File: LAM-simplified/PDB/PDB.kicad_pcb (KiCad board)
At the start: 2 copper layers, 115 x 115 mm, 22 parts, among them J1 Conn_02x03_Counter_Clockwise, J10 Conn_01x02, J11 Conn_01x02, J12 Conn_01x02, J13 Conn_01x02, J14 Conn_01x02, J15 Conn_01x02, J16 Conn_01x02, J2 Conn_02x03_Counter_Clockwise, J3 Conn_02x03_Counter_Clockwise, J4 Conn_02x03_Counter_Clockwise, J5 Conn_01x02, J6 Conn_01x02, J7 Conn_01x02, J8 Conn_01x02, J9 Conn_01x02

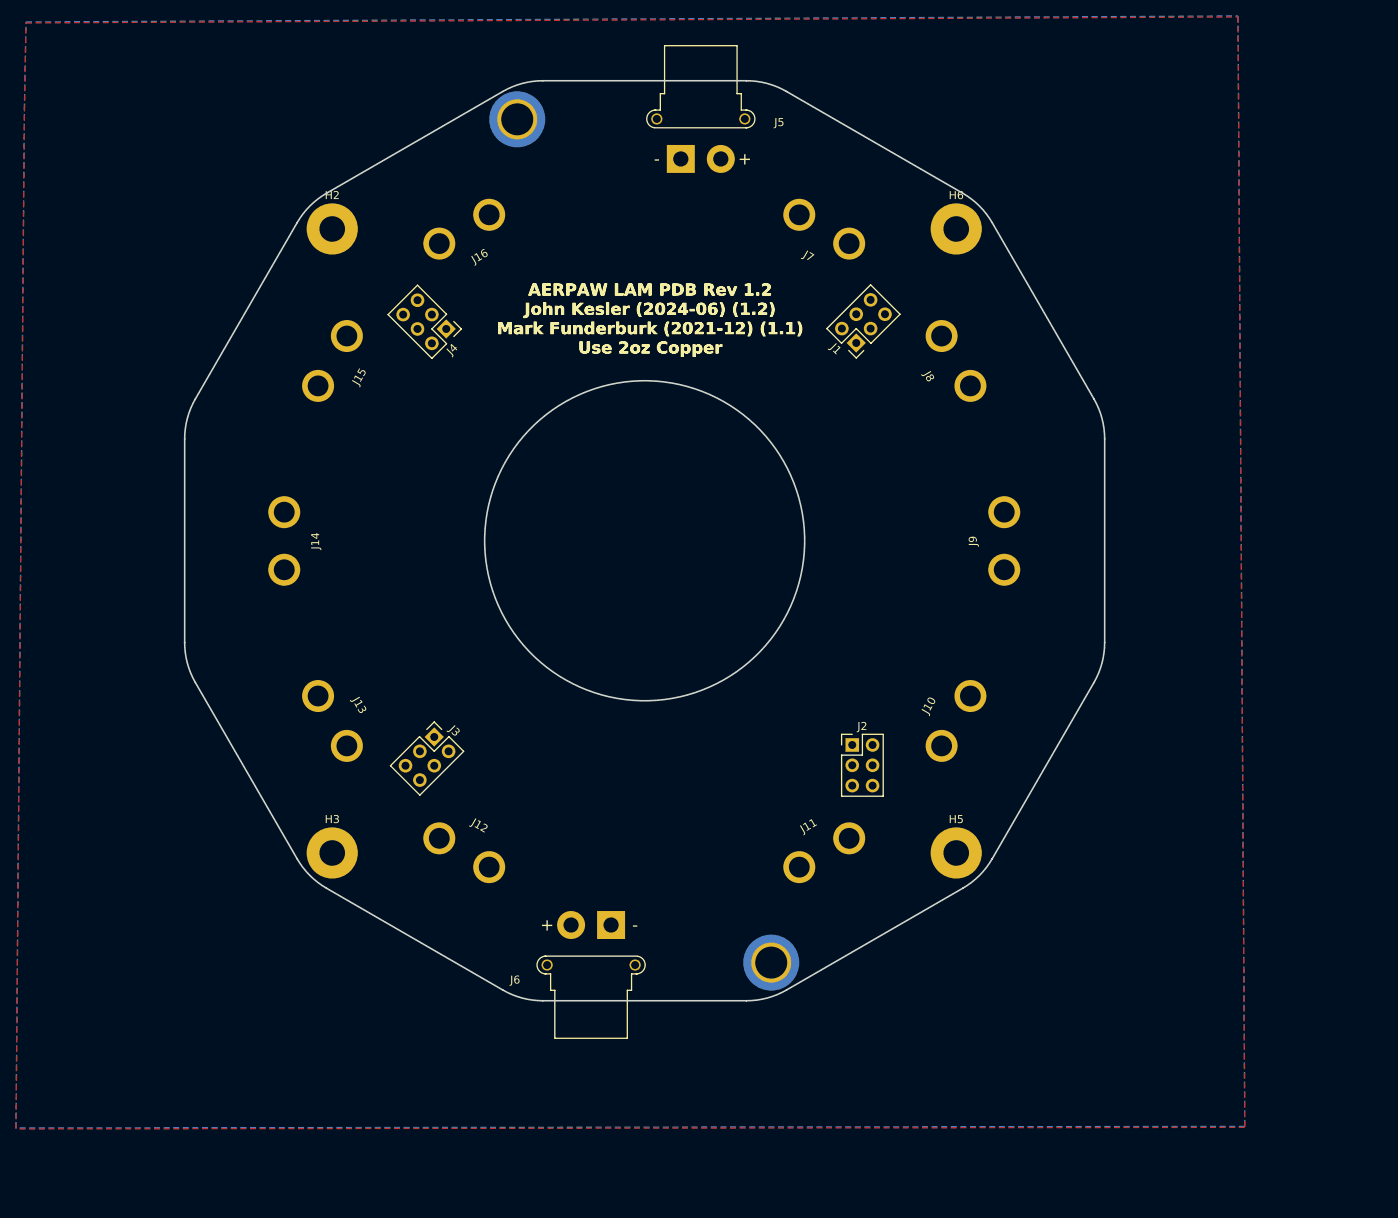
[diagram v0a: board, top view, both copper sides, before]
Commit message: update LAM PDB PCB r1.3
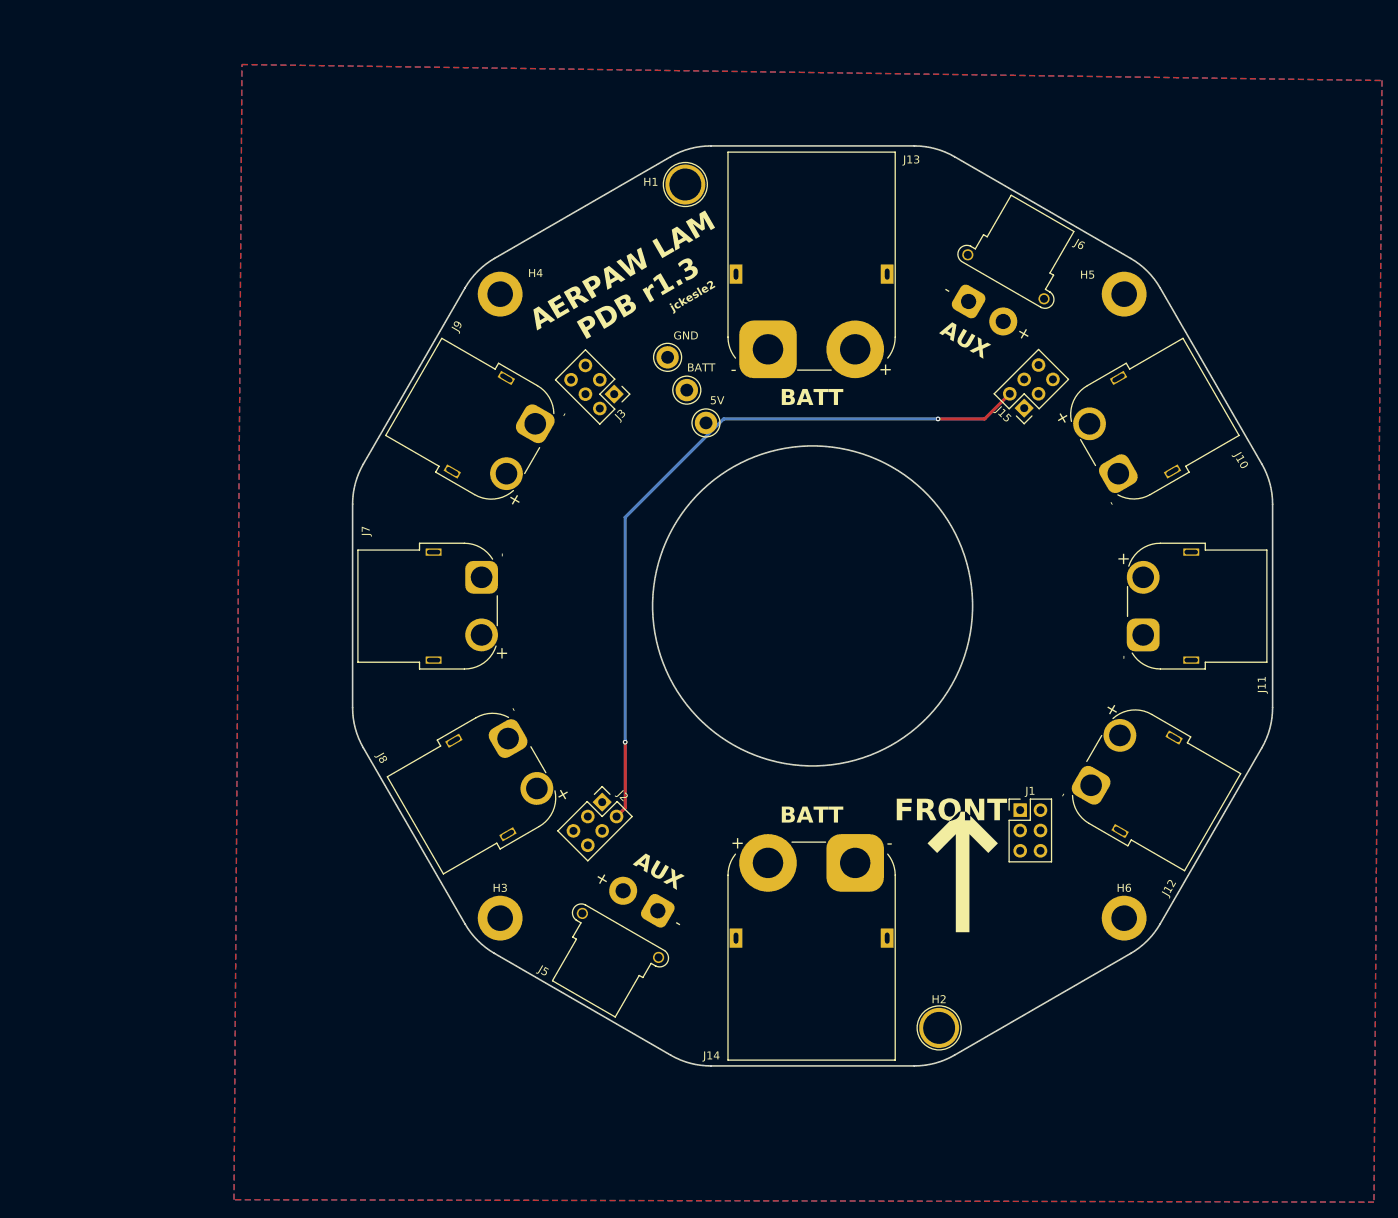
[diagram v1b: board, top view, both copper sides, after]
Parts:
- removed J16: Conn_01x02, PDB:XT-60_horizontal
- removed J4: Conn_02x03_Counter_Clockwise, PDB:PinSocket_2x03_P2.54mm_Vertical
- added 5V: TestPoint_Flag, TestPoint:TestPoint_Keystone_5010-5014_Multipurpose, F.Cu at (150.5, 74.7)
- added BATT: TestPoint_Flag, TestPoint:TestPoint_Keystone_5010-5014_Multipurpose, F.Cu at (148.1, 70.6)
- added GND: TestPoint_Flag, TestPoint:TestPoint_Keystone_5010-5014_Multipurpose, F.Cu at (145.7, 66.5)
- H1: value MountingHole_Pad -> M4; footprint PDB:MountingHole_4mm_Pad -> TestPoint:TestPoint_Plated_Hole_D4.0mm; moved to F.Cu
- H2: value MountingHole_Pad -> M4; footprint MountingHole:MountingHole_3.2mm_M3_Pad -> TestPoint:TestPoint_Plated_Hole_D4.0mm
- H3, H5, H6: value MountingHole_Pad -> M3; footprint MountingHole:MountingHole_3.2mm_M3_Pad -> MountingHole:MountingHole_3.2mm_M3_DIN965_Pad
- H4: value MountingHole_Pad -> M3; footprint PDB:MountingHole_4mm_Pad -> MountingHole:MountingHole_3.2mm_M3_DIN965_Pad; moved to F.Cu
- J1, J2, J3: value Conn_02x03_Counter_Clockwise -> 2.54mm 2x3; footprint PDB:PinSocket_2x03_P2.54mm_Vertical -> Connector_PinHeader_2.54mm:PinHeader_2x03_P2.54mm_Vertical
- J10, J11, J12, J7, J8, J9: value Conn_01x02 -> xt60-female; footprint PDB:XT-60_horizontal -> Connector_AMASS:AMASS_XT60PW-F_1x02_P7.20mm_Horizontal
- J13, J14: value Conn_01x02 -> xt90-female; footprint PDB:XT-60_horizontal -> Connector_AMASS:AMASS_XT90PW-M_1x02_P10.90mm_Horizontal
- J15: value Conn_01x02 -> 2.54mm 2x3; footprint PDB:XT-60_horizontal -> Connector_PinHeader_2.54mm:PinHeader_2x03_P2.54mm_Vertical
- J5, J6: value Conn_01x02 -> xt30-female; footprint P2_PowerSystem:AMASS_XT30PW-F_1x02_P2.50mm_Horizontal -> Connector_AMASS:AMASS_XT30PW-F_1x02_P2.50mm_Horizontal
- moved H2 125.4 mm to (179.6, 150.3)
- moved J5 94.0 mm to (144.5, 135.7), turned to 150 degrees
- moved H4 90.2 mm to (124.8, 58.6)
- moved J6 89.8 mm to (183.3, 59.5), turned to -30 degrees
- moved J15 89.4 mm to (190.3, 72.9), turned to 135 degrees
- moved H6 88.7 mm to (202.8, 136.6)
- moved J14 84.6 mm to (169.1, 129.7), turned to 180 degrees
- moved J12 80.6 mm to (198.6, 120.0), turned to -120 degrees
- moved J8 76.2 mm to (125.8, 114.2)
- moved J13 74.5 mm to (158.2, 65.5), turned to 0 degrees
- moved H5 72.9 mm to (202.8, 58.6)
- moved J7 64.0 mm to (122.5, 94.0), turned to 90 degrees
- moved J9 63.3 mm to (129.2, 74.8), turned to 60 degrees
- moved J1 61.9 mm to (189.8, 123.1), turned to 0 degrees
- moved J11 48.6 mm to (205.2, 101.2), turned to -90 degrees
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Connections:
- J1 pad 1: V+_BATT -> /vbat
- J1 pad 2: +5VA -> /vbat
- J10 pad 1: V+_BATT -> GND
- J10 pad 2: GND -> /vbat
- J11 pad 1: V+_BATT -> GND
- J11 pad 2: GND -> /vbat
- J12 pad 1: V+_BATT -> GND
- J12 pad 2: GND -> /vbat
- J13 pad 1: V+_BATT -> GND
- J13 pad 2: GND -> /vbat
- J14 pad 1: V+_BATT -> GND
- J14 pad 2: GND -> /vbat
- J15 pad 1: V+_BATT -> /vbat
- J15 pad 2: GND -> +5V
- J2 pad 1: V+_BATT -> /vbat
- J2 pad 2: V+_BATT -> +5V
- J2 pad 6: GND -> /vbat
- J3 pad 1: V+_BATT -> /vbat
- J3 pad 2: +5VA -> /vbat
- J3 pad 6: V+_BATT -> /vbat
- J5 pad 2: V+_BATT -> /vbat
- J6 pad 2: V+_BATT -> /vbat
- J7 pad 1: V+_BATT -> GND
- J7 pad 2: GND -> /vbat
- J8 pad 1: V+_BATT -> GND
- J8 pad 2: GND -> /vbat
- J9 pad 1: V+_BATT -> GND
- J9 pad 2: GND -> /vbat
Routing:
- net +5V: track 0.00 -> 92.3 mm, vias 0 -> 2
- added copper zone on F.Cu, net /vbat
- added copper zone on B.Cu, net GND
- removed copper zone on F.Cu, net GND
- removed copper zone on B.Cu, net V+_BATT
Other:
- board text added: "AERPAW LAM PDB r1.3"
- board text added: "AUX"
- board text added: "BATT"
- board text added: "FRONT"
- board text added: "jckesle2"
- board text added: "↑"
- board text removed: "AERPAW LAM PDB Rev 1.2 John Kesler (2024-06) (1.2) Mark Funderburk (2021-12) (1.1) Use 2oz Copper"
